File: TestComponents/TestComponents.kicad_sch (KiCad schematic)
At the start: 15 parts, among them J5 RFShield_OnePiece, J6 RFShield_OnePiece, U1 AD7991

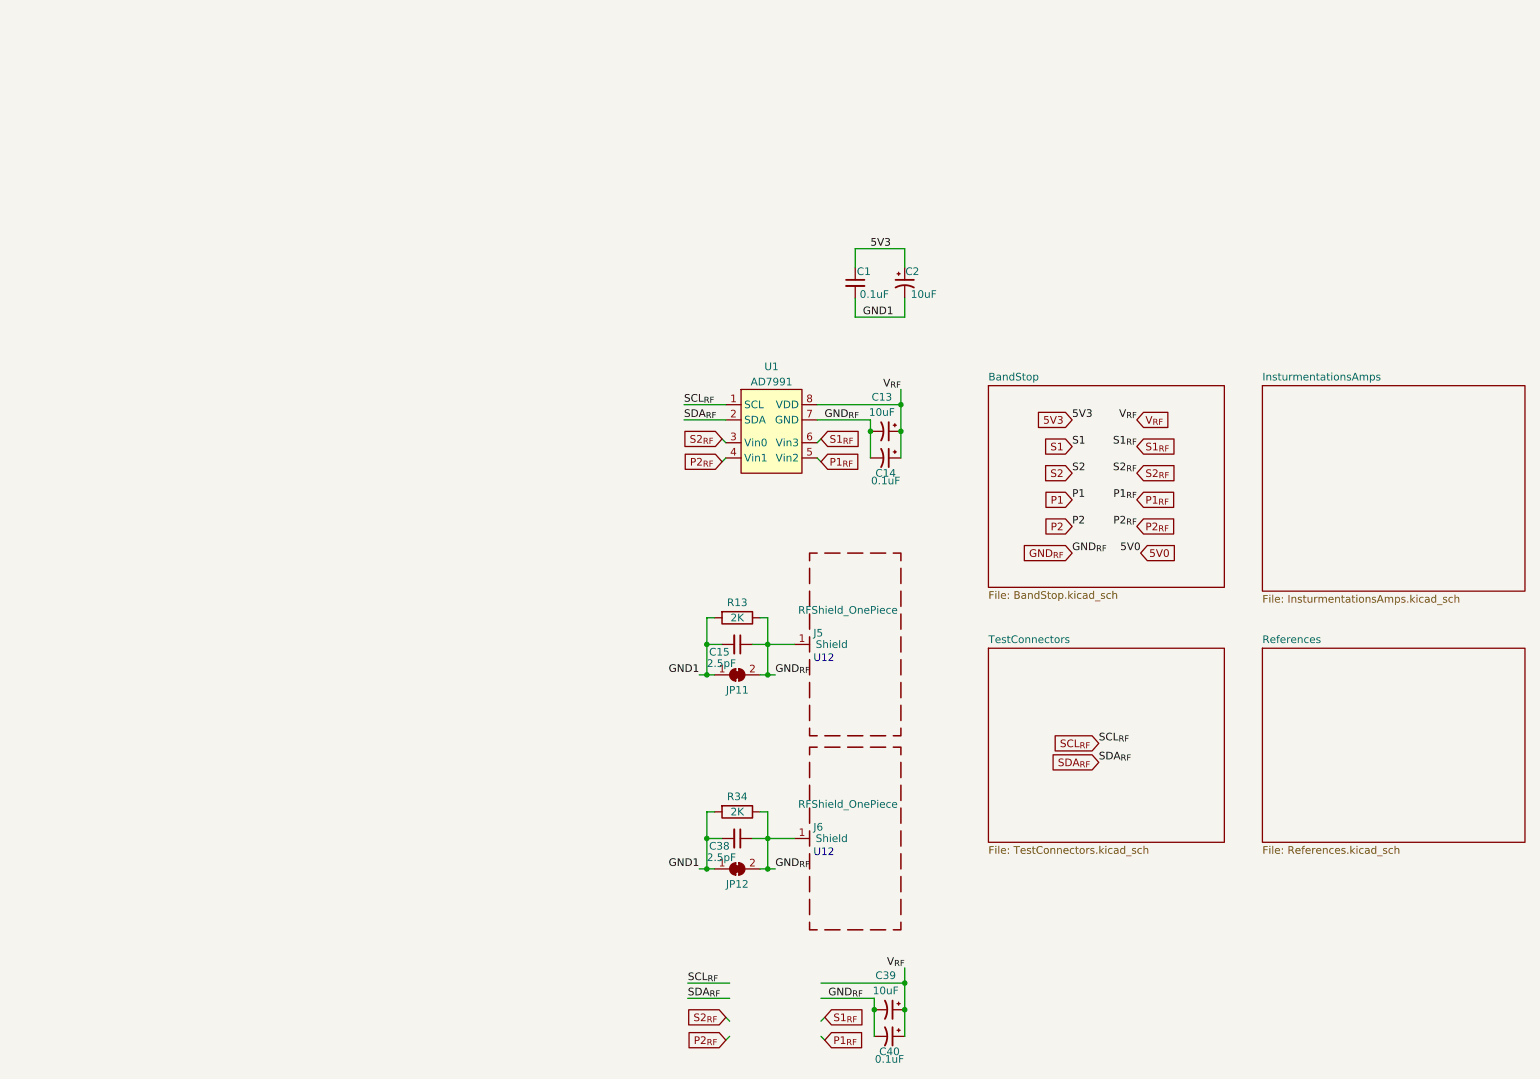
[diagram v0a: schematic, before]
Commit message: SpectDrone Development
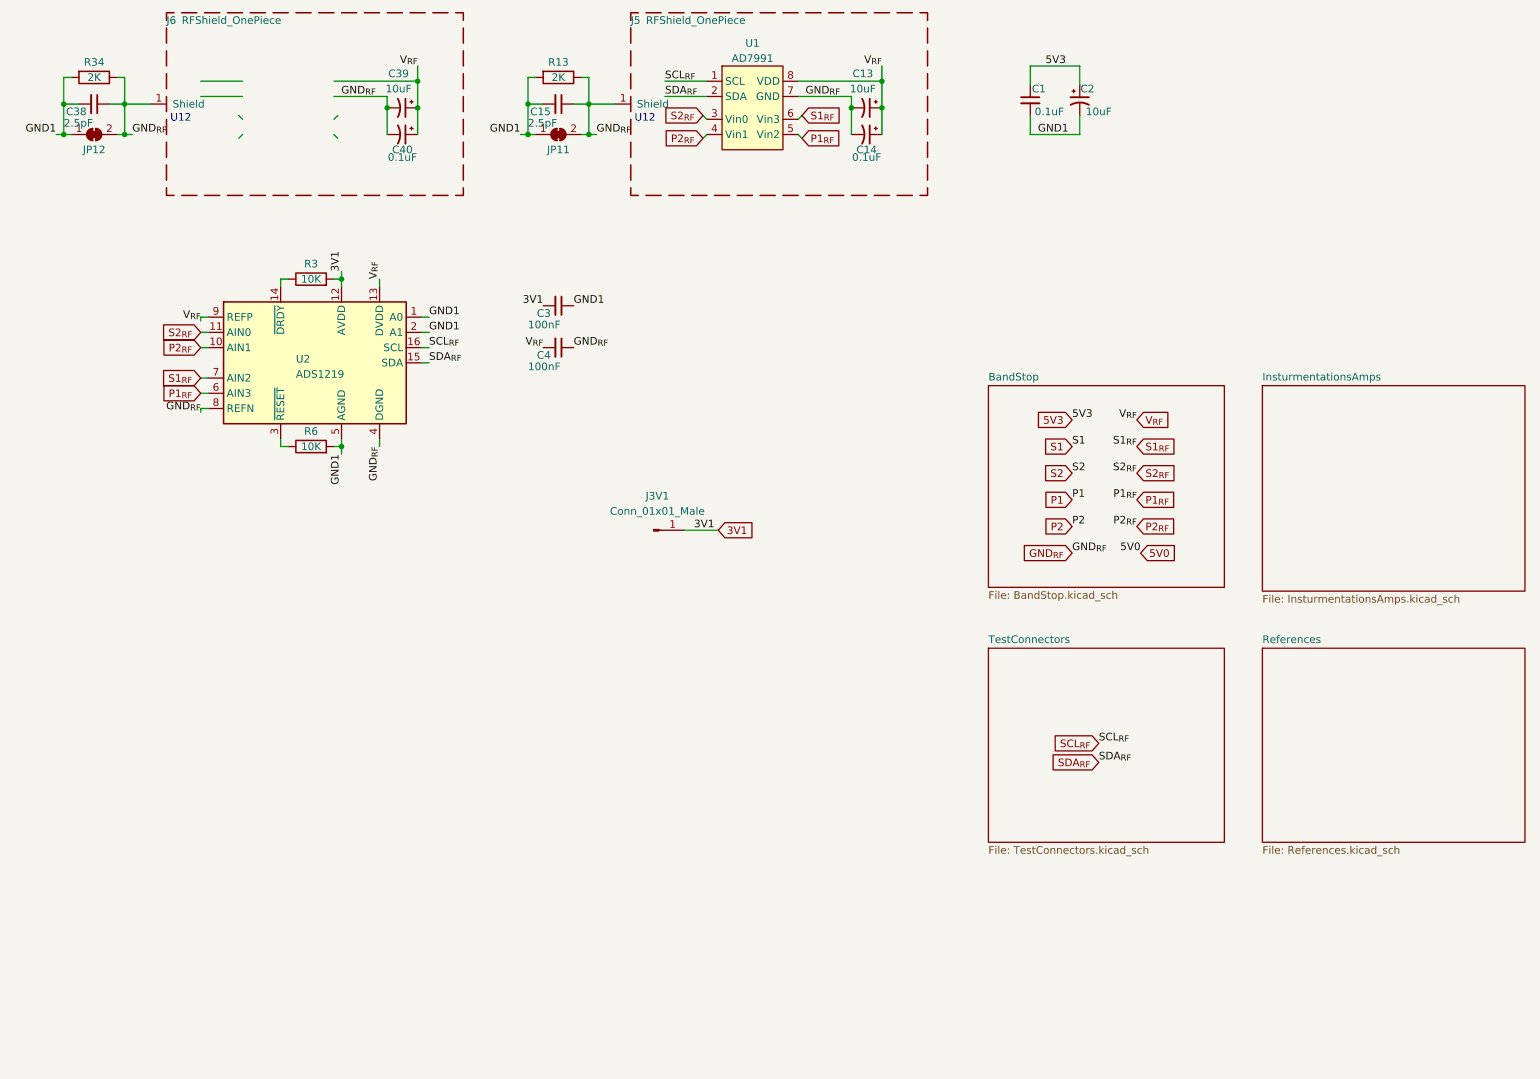
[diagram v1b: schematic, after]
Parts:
- added C3, C4: 100nF, Capacitor_SMD:C_0805_2012Metric, symbol Device:C_Small
- added J3V1: Conn_01x01_Male, symbol Connector:Conn_01x01_Male
- added R3, R6: 10K, symbol Device:R
- added U2: ADS1219, Package_SO:TSSOP-16_4.4x5mm_P0.65mm, symbol ads1219:ADS1219
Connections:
- net GND1: now also C3.1, R6.2, U2.1 (A0), U2.2 (A1), U2.5 (AGND)
- net GND_{RF}: now also C4.1, U2.4 (DGND), U2.8 (REFN)
- net P1_{RF}: now also U2.6 (AIN3)
- net P2_{RF}: now also U2.10 (AIN1)
- net S1_{RF}: now also U2.7 (AIN2)
- net S2_{RF}: now also U2.11 (AIN0)
- net SCL_{RF}: now also U2.16 (SCL)
- net SDA_{RF}: now also U2.15 (SDA)
- net V_{RF}: now also C4.2, U2.13 (DVDD), U2.9 (REFP)
- new net: R3.1, U2.14 (~{DRDY})
- new net: R6.1, U2.3 (~{RESET})
- new net 3V1: C3.2, J3V1.1 (Pin_1), R3.2, U2.12 (AVDD)
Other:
- moved on the sheet: C1, C13, C14, C15, C2, C38, C39, C40, JP11, JP12, R13, R34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

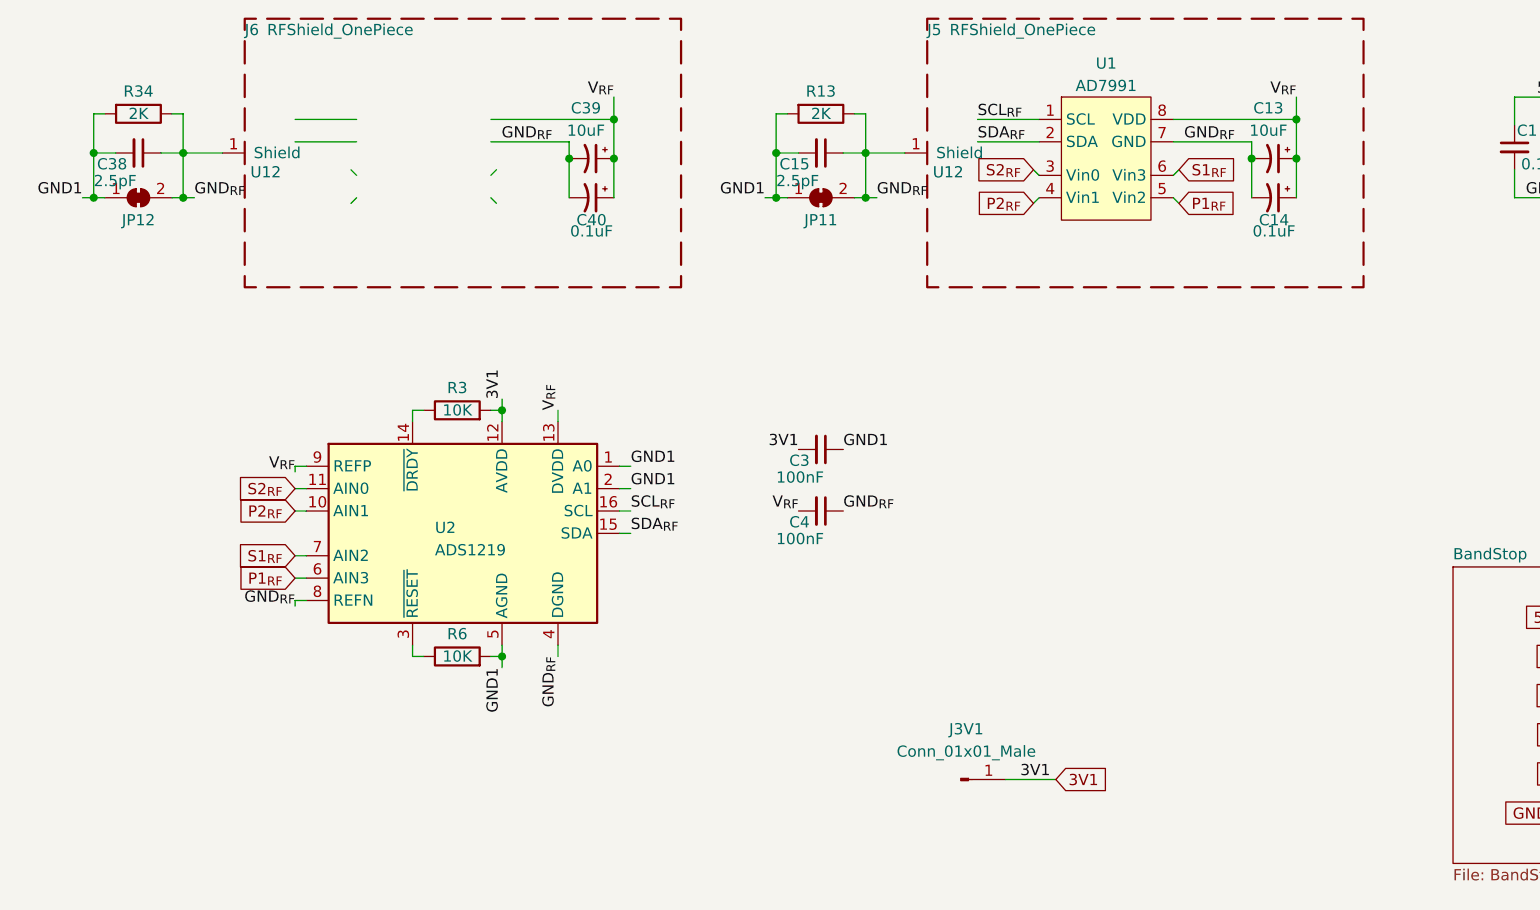
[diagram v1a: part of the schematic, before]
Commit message: SpectDrone Development
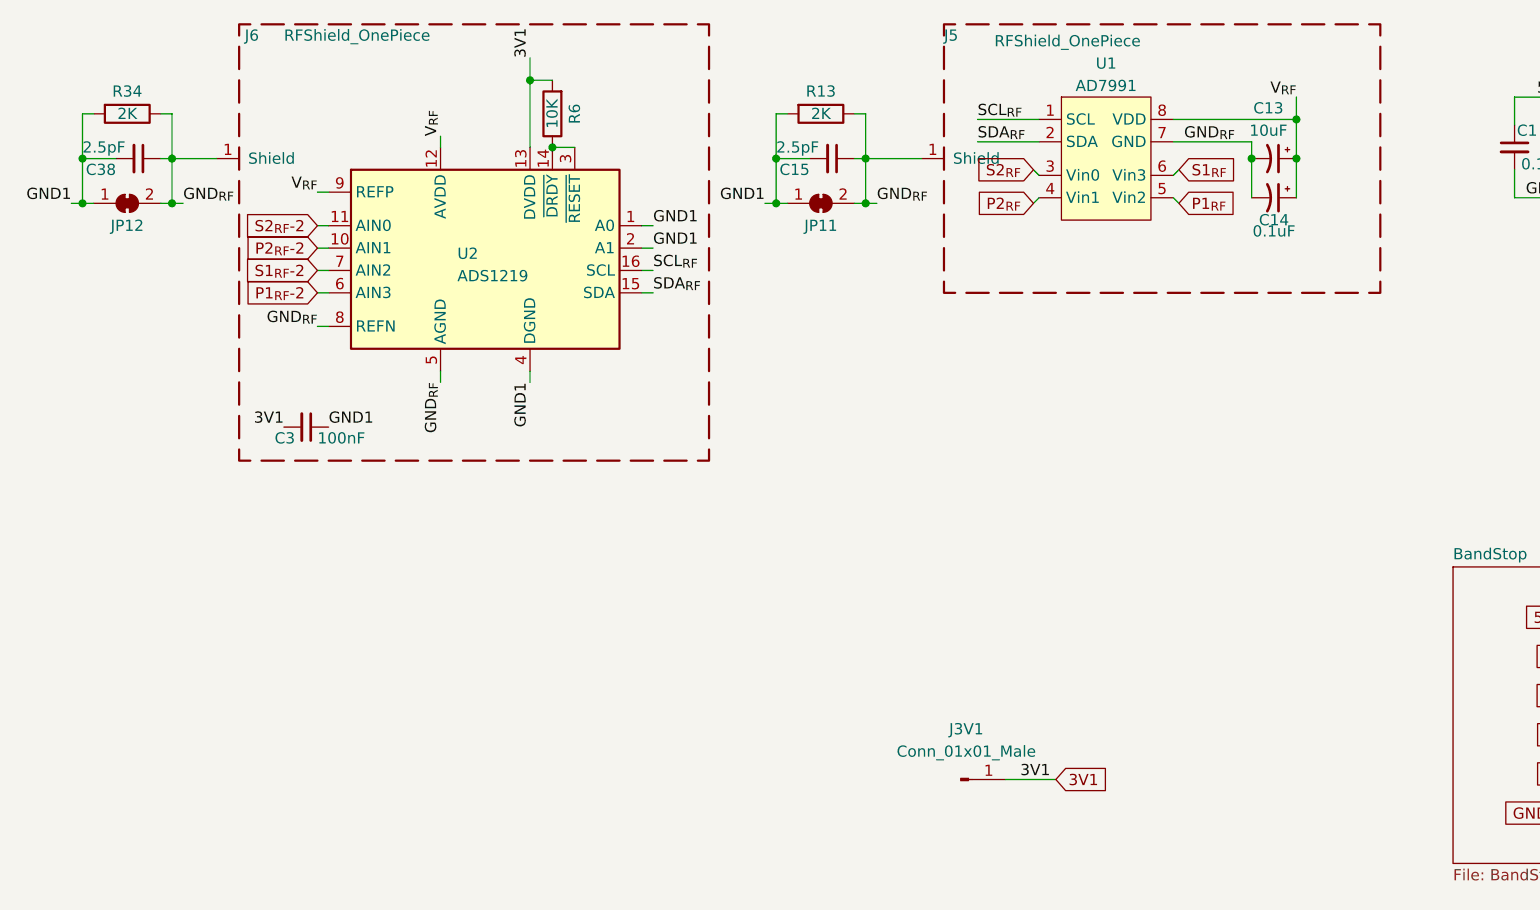
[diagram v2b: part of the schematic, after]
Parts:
- removed C39: 10uF, Capacitor_SMD:C_0805_2012Metric, symbol Device:C_Polarized_Small_US
- removed C4: 100nF, Capacitor_SMD:C_0805_2012Metric, symbol Device:C_Small
- removed C40: 0.1uF, Capacitor_SMD:C_0603_1608Metric, symbol Device:C_Polarized_Small_US
- removed R3: 10K, symbol Device:R
- R13, R34: footprint Capacitor_SMD:C_0805_2012Metric -> Resistor_SMD:R_0805_2012Metric
- R6: footprint (none) -> Resistor_SMD:R_0805_2012Metric
- U2: symbol ads1219:ADS1219 -> ADS1219:ADS1219
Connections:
- net 3V1: now also R6.2, U2.13 (DVDD); no longer U2.12 (AVDD)
- net GND1: now also U2.4 (DGND); no longer R6.2, U2.5 (AGND)
- net GND_{RF}: now also U2.5 (AGND); no longer U2.4 (DGND)
- net P1_{RF}: no longer U2.6 (AIN3)
- net P2_{RF}: no longer U2.10 (AIN1)
- net S1_{RF}: no longer U2.7 (AIN2)
- net S2_{RF}: no longer U2.11 (AIN0)
- net V_{RF}: now also U2.12 (AVDD); no longer U2.13 (DVDD)
- net at U2.14 (~{DRDY}): now also R6.1, U2.3 (~{RESET})
- new net P1_{RF}-2: U2.6 (AIN3)
- new net P2_{RF}-2: U2.10 (AIN1)
- new net S1_{RF}-2: U2.7 (AIN2)
- new net S2_{RF}-2: U2.11 (AIN0)
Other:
- note removed: "U12"
- moved on the sheet: C15, C3, C38, J5, JP11, JP12, R34, R6, U2
